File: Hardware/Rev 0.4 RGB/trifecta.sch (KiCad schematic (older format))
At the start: 263 parts, among them J1 USB2_C_Receptacle, SW1 SW_Push, SW2 Rotary_Encoder_Switch, SW3 Rotary_Encoder_Switch, SW4 Rotary_Encoder_Switch, U1 ATmega32U4-AU, U2 SRV05-4, Y1 16MHz

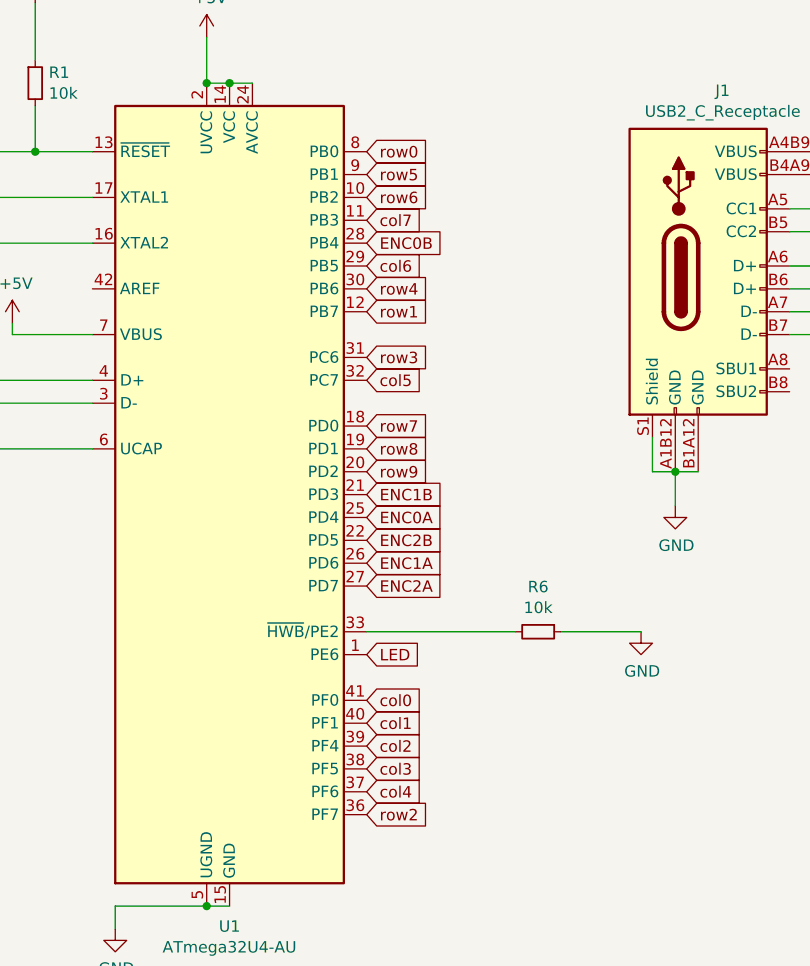
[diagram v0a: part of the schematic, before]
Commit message: 8/3/2020
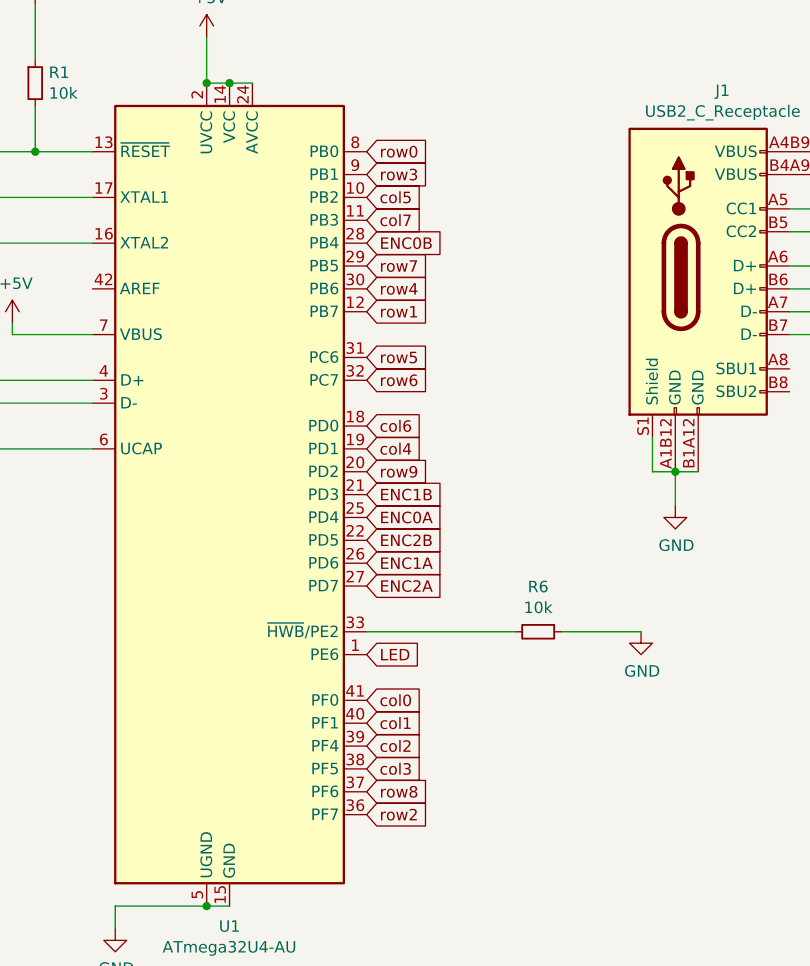
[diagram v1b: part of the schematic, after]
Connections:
- net col4: now also U1.19 (PD1); no longer U1.37 (PF6)
- net col5: now also U1.10 (PB2); no longer U1.32 (PC7)
- net col6: now also U1.18 (PD0); no longer U1.29 (PB5)
- net row3: now also U1.9 (PB1); no longer U1.31 (PC6)
- net row5: now also U1.31 (PC6); no longer U1.9 (PB1)
- net row6: now also U1.32 (PC7); no longer U1.10 (PB2)
- net row7: now also U1.29 (PB5); no longer U1.18 (PD0)
- net row8: now also U1.37 (PF6); no longer U1.19 (PD1)
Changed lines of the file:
@@
 Text GLabel 5500 3400 2    50   Input ~ 0
 ENC0B
-Text GLabel 5500 3500 2    50   Input ~ 0
+Text GLabel 5500 4200 2    50   Input ~ 0
 col6
 Text GLabel 5500 3600 2    50   Input ~ 0
@@
 Text GLabel 5500 3700 2    50   Input ~ 0
 row1
-Text GLabel 5500 3900 2    50   Input ~ 0
+Text GLabel 5500 3100 2    50   Input ~ 0
 row3
-Text GLabel 5500 4000 2    50   Input ~ 0
+Text GLabel 5500 3200 2    50   Input ~ 0
 col5
 Text GLabel 5500 4600 2    50   Input ~ 0
@@
 Text GLabel 5500 5700 2    50   Input ~ 0
 col3
-Text GLabel 5500 5800 2    50   Input ~ 0
+Text GLabel 5500 4300 2    50   Input ~ 0
 col4
 Text GLabel 5500 5900 2    50   Input ~ 0
@@
 Text GLabel 3775 13125 0    50   Input ~ 0
 row9
-Text GLabel 5500 3100 2    50   Input ~ 0
+Text GLabel 5500 3900 2    50   Input ~ 0
 row5
-Text GLabel 5500 3200 2    50   Input ~ 0
+Text GLabel 5500 4000 2    50   Input ~ 0
 row6
-Text GLabel 5500 4200 2    50   Input ~ 0
+Text GLabel 5500 3500 2    50   Input ~ 0
 row7
-Text GLabel 5500 4300 2    50   Input ~ 0
+Text GLabel 5500 5800 2    50   Input ~ 0
 row8
 Text GLabel 5500 4400 2    50   Input ~ 0
